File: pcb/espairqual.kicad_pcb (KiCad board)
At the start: 2 copper layers, 81 x 44.8 mm, 38 parts, among them J1 24VAC, J2 PMSX003, J3 USB_C_Receptacle_USB2.0, J7 eflashy32, U1 BD9G101G, U2 ESP32-WROOM-32D, U3 AMS1117-3.3

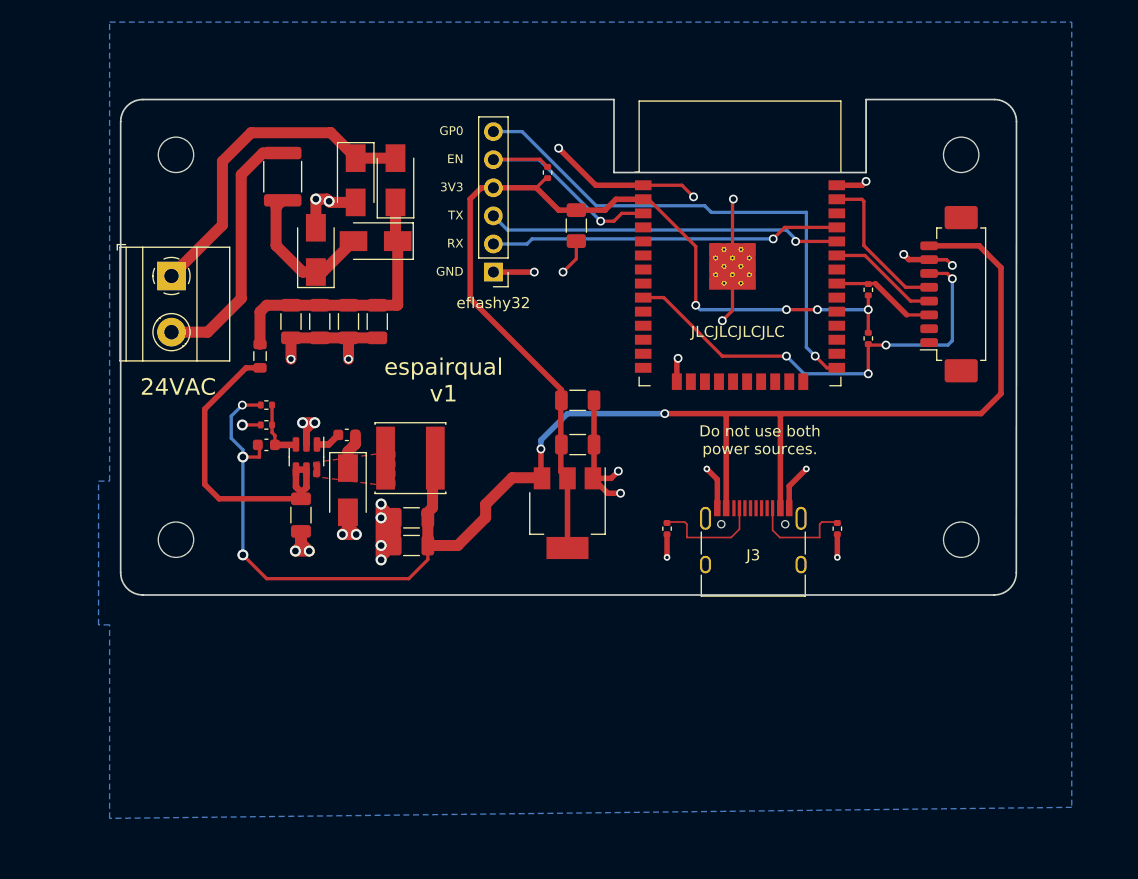
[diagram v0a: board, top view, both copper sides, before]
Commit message: update workflow
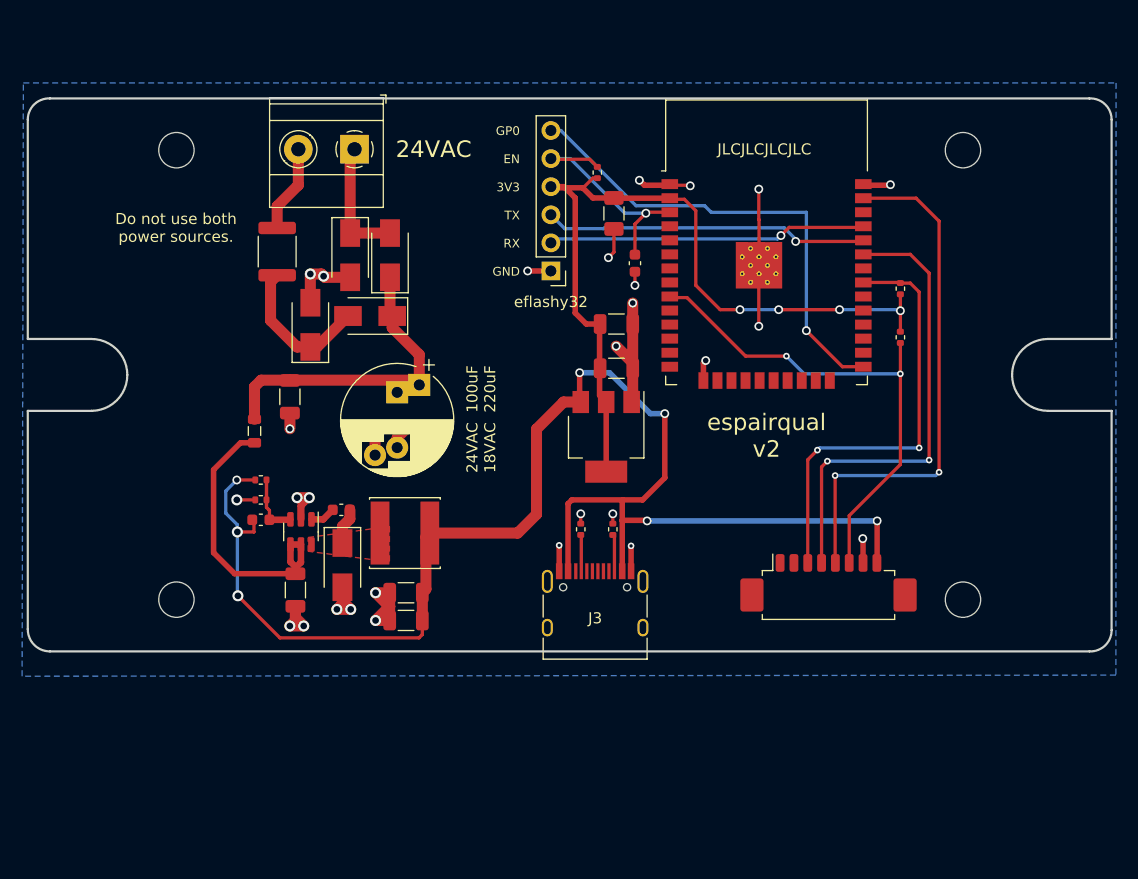
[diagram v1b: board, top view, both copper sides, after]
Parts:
- removed C11, C12: 10uF 50V, Capacitor_SMD:C_1206_3216Metric
- removed REF** (x4): MountingHole_3.2mm_M3, MountingHole:MountingHole_3.2mm_M3
- added C16: 1uF, Capacitor_SMD:C_0603_1608Metric, F.Cu at (71.5, 44.8)
- added H1: MountingHole, MountingHole:MountingHole_3.2mm_M3, F.Cu at (30.0, 75.2)
- added H2: MountingHole, MountingHole:MountingHole_3.2mm_M3, F.Cu at (101.2, 75.2)
- added H3: MountingHole, MountingHole:MountingHole_3.2mm_M3, F.Cu at (30.0, 34.6)
- added H4: MountingHole, MountingHole:MountingHole_3.2mm_M3, F.Cu at (101.2, 34.6)
- C10: value 10uF 50V -> 100uF 50V; footprint Capacitor_SMD:C_1206_3216Metric -> Capacitor_THT:CP_Radial_D10.0mm_P5.00mm_P7.50mm
- moved J2 29.1 mm to (89.0, 74.3), turned to 0 degrees
- moved R7 20.3 mm to (69.5, 68.9), turned to 90 degrees
- moved J1 20.1 mm to (46.1, 34.5), turned to 180 degrees
- moved J3 15.4 mm to (67.9, 76.7)
- moved C10 9.48 mm to (50.0, 56.5)
- moved C6 8.62 mm to (40.3, 56.9)
- moved R4 7.80 mm to (66.6, 68.9), turned to 90 degrees
- moved C8 7.74 mm to (69.8, 54.3)
- moved C9 7.74 mm to (69.8, 50.3)
- moved U3 7.74 mm to (68.9, 60.5)
- moved D3 6.79 mm to (47.5, 49.6)
- moved D4 6.79 mm to (45.8, 44.1)
- moved D5 6.79 mm to (49.4, 44.1)
- moved L1 6.79 mm to (50.7, 69.2)
- moved R12 6.79 mm to (37.7, 64.4)
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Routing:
- net /PMS_RXD: track 14.0 -> 47.8 mm, vias 0 -> 2
- net GND: track 121.0 -> 87.3 mm, vias 31 -> 30
- net /PMS_TXD: track 10.1 -> 42.2 mm, vias 0 -> 2
- net /PMS_RESET: track 9.52 -> 39.4 mm, vias 0 -> 2
- net Net-(D4-Pad1): track 30.0 -> 11.3 mm
- net Net-(F1-Pad1): track 23.3 -> 7.91 mm
- net +3V3: track 84.9 -> 74.6 mm
- net +5V: track 141.4 -> 131.7 mm, vias 5 -> 7
- net Net-(J3-PadA5): track 10.5 -> 2.57 mm
- net Net-(J3-PadB5): track 9.83 -> 2.61 mm
- net /Vrec: track 25.0 -> 29.1 mm
- net /PMS_SET: track 41.6 -> 45.6 mm, vias 4 -> 2
- net /GPIO0: track 47.0 -> 43.4 mm
- net /RX: track 31.7 -> 28.9 mm
- net /TX: track 32.1 -> 29.5 mm
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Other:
- board size 81 x 44.8 mm -> 98 x 50 mm
- board text added: "24VAC 100uF 18VAC 220uF"
- board text added: "Hammond 1593"
- board text added: "espairqual v2"
- board text removed: "espairqual v1"

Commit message: changes
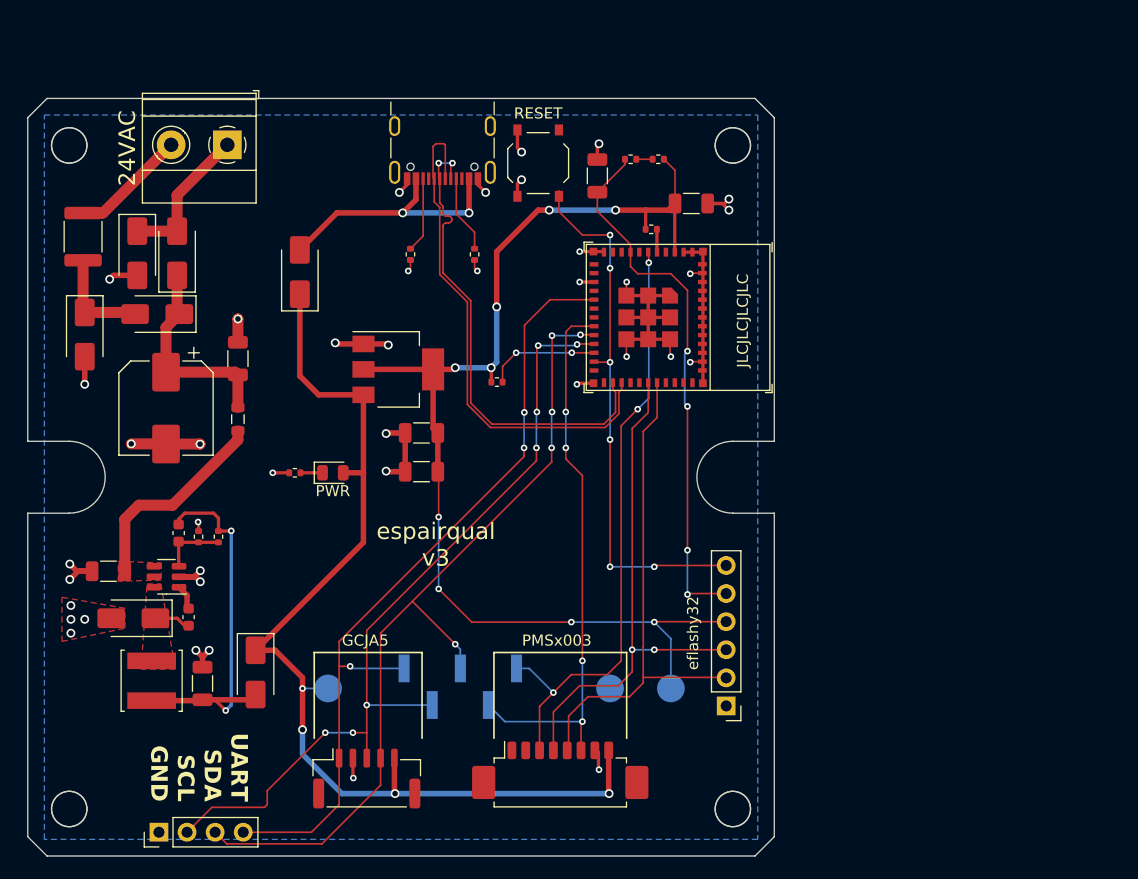
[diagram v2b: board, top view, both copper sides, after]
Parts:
- removed C16: 1uF, Capacitor_SMD:C_0603_1608Metric
- removed C2, C3: 47u, Capacitor_SMD:C_1206_3216Metric
- removed R7: 5k1, Resistor_SMD:R_0402_1005Metric
- removed U2: ESP32-WROOM-32D, RF_Module:ESP32-WROOM-32
- added C11: 10uF 50V, Capacitor_SMD:C_1206_3216Metric, F.Cu at (76.6, 39.4)
- added C12: 10uF 50V, Capacitor_SMD:C_1206_3216Metric, F.Cu at (68.1, 36.9)
- added D6: SS210, Diode_SMD:D_SMA, F.Cu at (41.2, 45.6)
- added D7: SS210, Diode_SMD:D_SMA, F.Cu at (37.2, 81.8)
- added D8: PWR, LED_SMD:LED_0805_2012Metric, F.Cu at (44.2, 63.8)
- added J4: USBC, Connector_USB:USB_C_Receptacle_GCT_USB4105-xx-A_16P_TopMnt_Horizontal, F.Cu at (54.1, 33.5)
- added J5: GCJA5, Connector_JST:JST_GH_SM05B-GHS-TB_1x05-1MP_P1.25mm_Horizontal, F.Cu at (47.2, 91.4)
- added J6: TEST, Connector_PinHeader_2.54mm:PinHeader_1x04_P2.54mm_Vertical, F.Cu at (28.5, 96.2)
- added R10: 5k1, Resistor_SMD:R_0402_1005Metric, F.Cu at (57.0, 44.0)
- added R11: 5k1, Resistor_SMD:R_0402_1005Metric, F.Cu at (51.2, 44.0)
- added R6: 680, Resistor_SMD:R_0402_1005Metric, F.Cu at (40.8, 63.8)
- added SW1: RESET, Button_Switch_SMD:SW_Push_1P1T_XKB_TS-1187A, F.Cu at (62.8, 35.8)
- added TP1: +5V, TestPoint:TestPoint_Pad_D2.5mm, B.Cu at (43.8, 83.2)
- added TP2: GND, TestPoint:TestPoint_Pad_D2.5mm, B.Cu at (69.2, 83.2)
- added TP3: +3.3V, TestPoint:TestPoint_Pad_D2.5mm, B.Cu at (74.8, 83.2)
- added U4: ESP32-C3-MINI-1, Espressif:ESP32-C3-MINI-1, F.Cu at (75.4, 49.7)
- C1, C7, C8, C9: value 10u -> 10uF 50V
- C10: footprint Capacitor_THT:CP_Radial_D10.0mm_P5.00mm_P7.50mm -> Capacitor_SMD:CP_Elec_8x10
- J3: value USB_C_Receptacle_USB2.0 -> eflashy32; footprint Connector_USB:USB_C_Receptacle_HRO_TYPE-C-31-M-12 -> Connector_PinHeader_2.54mm:PinHeader_1x06_P2.54mm_Vertical
- J7: value eflashy32 -> AUX; footprint Connector_PinHeader_2.54mm:PinHeader_1x06_P2.54mm_Vertical -> Connector_PinHeader_2.54mm:PinHeader_1x05_P2.54mm_Vertical_SMD_Pin1Left; moved to B.Cu
- L1: footprint Inductor_SMD:L_Sunlord_SWPA60xxS -> Inductor_SMD:L_Sunlord_SWPA5012S
- R1, R3, R5: value 10K -> 5k1
- moved C7 56.5 mm to (32.4, 82.8)
- moved J7 38.5 mm to (55.7, 83.1), turned to -90 degrees
- moved J2 29.6 mm to (64.8, 91.2)
- moved H2 28.1 mm to (80.3, 94.2)
- moved R4 27.9 mm to (73.0, 41.7), turned to 0 degrees
- moved R3 27.2 mm to (73.6, 35.4), turned to 180 degrees
- moved R1 27.1 mm to (71.1, 35.4), turned to 180 degrees
- moved L1 26.5 mm to (27.8, 82.6), turned to -90 degrees
- moved H1 21.3 mm to (20.4, 94.2)
- moved R5 21.0 mm to (59.0, 55.5), turned to 0 degrees
- moved C10 20.9 mm to (29.1, 57.9)
- moved H4 20.8 mm to (80.3, 34.1)
- moved D2 20.4 mm to (21.8, 51.2), turned to -90 degrees
- moved C9 20.2 mm to (52.2, 60.1), turned to 180 degrees
- moved C8 20.0 mm to (52.2, 63.6), turned to 180 degrees
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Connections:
- C4 pad 1: +5V -> Net-(D7-A)
- C7 pad 1: GND -> Net-(D7-A)
- C7 pad 2: +3V3 -> GND
- J2 pad 3: /PMS_RESET -> /GPIO3
- J2 pad 6: /PMS_SET -> /GPIO5
- J7 pad 1: GND -> /GPIO10
- J7 pad 2: /RX -> /GPIO7
- J7 pad 3: /TX -> /GPIO6
- J7 pad 4: +3V3 -> /GPIO5
- J7 pad 5: /EN -> /GPIO3
- L1 pad 2: +5V -> Net-(D7-A)
- R1 pad 1: /PMS_RESET -> Net-(R1-Pad1)
- R1 pad 2: +3V3 -> /EN
- R12 pad 2: +5V -> Net-(D7-A)
- R3 pad 1: /PMS_SET -> +3V3
- R3 pad 2: +3V3 -> Net-(R1-Pad1)
- R4 pad 1: Net-(J3-PadA5) -> +3V3
- R4 pad 2: GND -> Net-(U4-GPIO2/ADC1_CH2)
- R5 pad 1: /EN -> +3V3
- R5 pad 2: +3V3 -> Net-(U4-GPIO8)
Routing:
- net /GPIO6: track 0.00 -> 76.3 mm, vias 0 -> 5
- net /GPIO7: track 0.00 -> 75.5 mm, vias 0 -> 7
- net /GPIO10: track 0.00 -> 73.2 mm, vias 0 -> 3
- net /GPIO3: track 0.00 -> 55.2 mm, vias 0 -> 3
- net /GPIO5: track 0.00 -> 50.4 mm, vias 0 -> 4
- net D+: track 0.00 -> 46.9 mm
- net /PMS_SET: track 45.6 -> 0.00 mm, vias 2 -> 0
- net D-: track 0.00 -> 43.8 mm, vias 0 -> 2
- net /PMS_RESET: track 39.4 -> 0.00 mm, vias 2 -> 0
- net +5V: track 131.7 -> 93.7 mm, vias 7 -> 4
- net Net-(D7-A): track 0.00 -> 34.6 mm, vias 0 -> 2
- net +3V3: track 74.6 -> 105.9 mm, vias 4 -> 9
- net /TX: track 29.5 -> 0.00 mm, vias 1 -> 0
- net /RX: track 28.9 -> 0.00 mm, vias 1 -> 0
- net /EN: track 21.5 -> 49.3 mm, vias 1 -> 4
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- added copper zone on F.Cu, net GND
- added copper zone on F.Cu, net Net-(U1-EN)
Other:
- board size 98 x 50 mm -> 67.5 x 68.5 mm
- board text added: "GCJA5"
- board text added: "GPIO10 GPIO GPIO3"
- board text added: "GPIO7 GPIO5"
- board text added: "Hammond 1593ARBK"
- board text added: "PMSx003"
- board text added: "UART SDA SCL GND"
- board text added: "espairqual v3"
- board text removed: "24VAC 100uF 18VAC 220uF"
- board text removed: "Do not use both power sources."
- board text removed: "GP0 EN 3V3 TX RX GND"
- board text removed: "Hammond 1593"
- board text removed: "espairqual v2"
